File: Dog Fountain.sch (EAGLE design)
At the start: 19 parts, among them IC1 L298, J1 22-27-2021-02, J4 22-27-2021-02

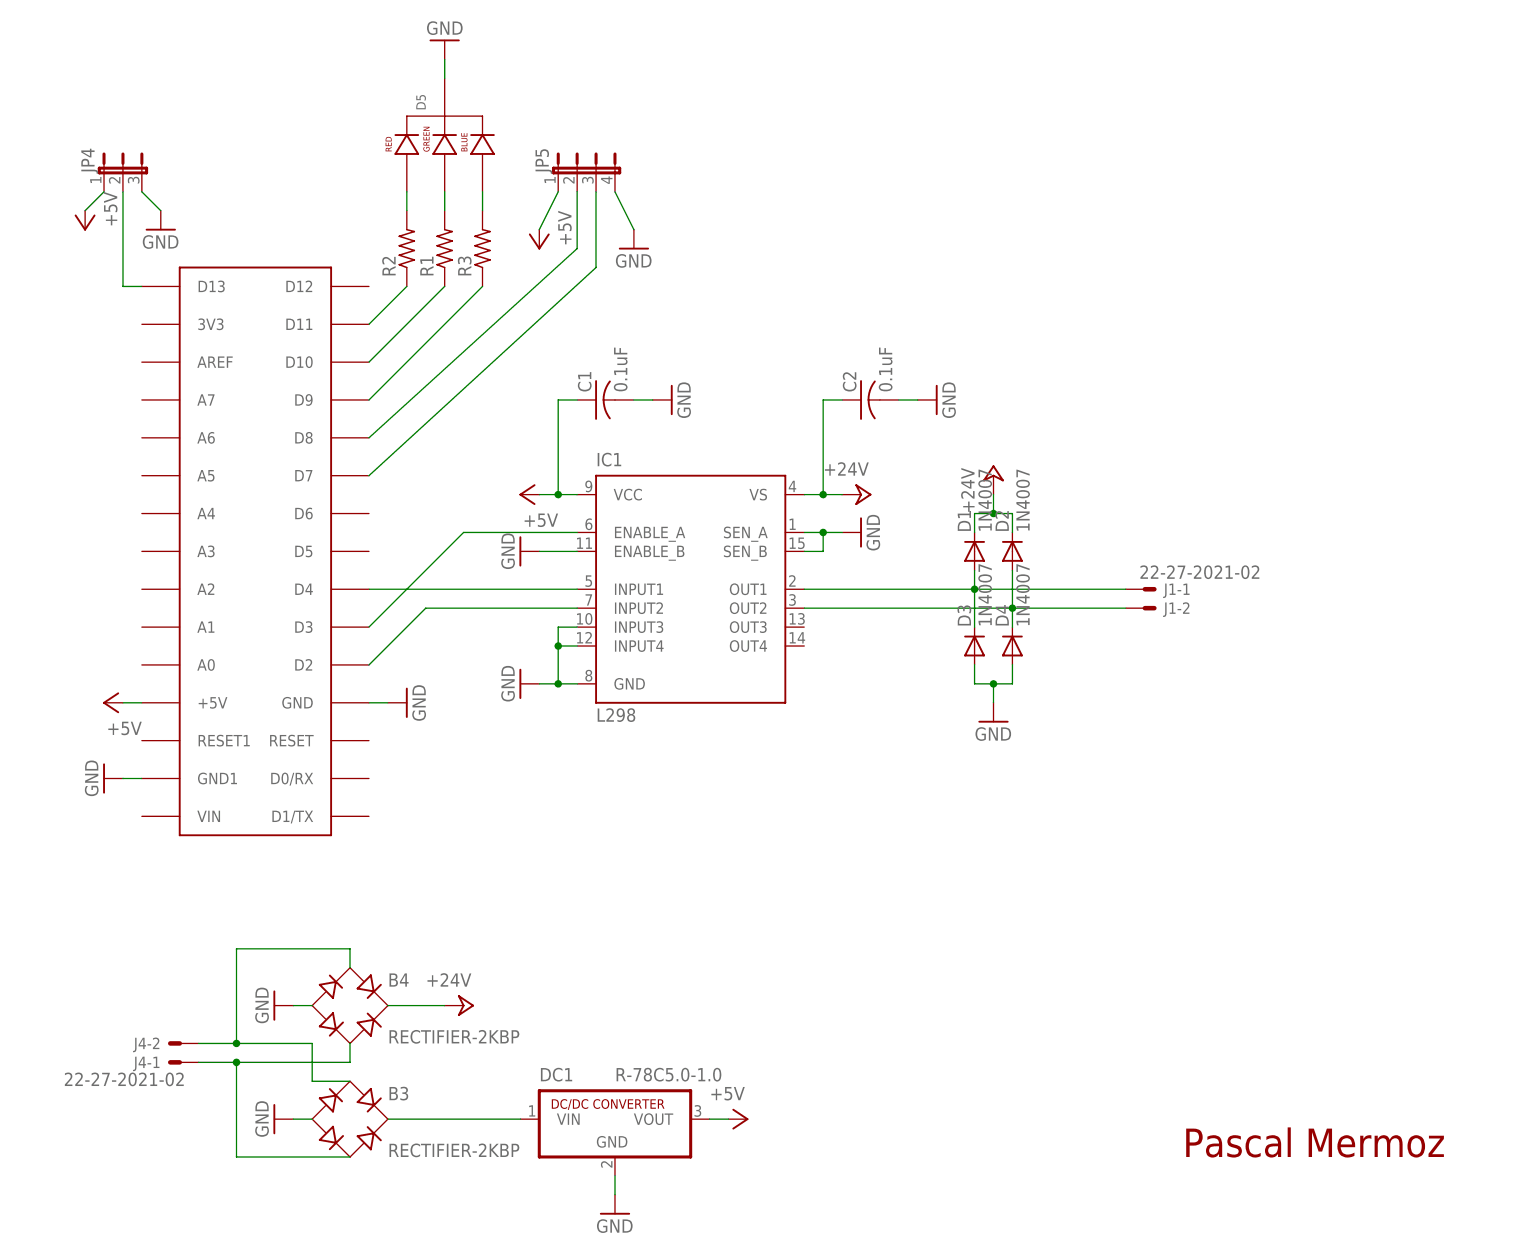
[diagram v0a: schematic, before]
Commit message: PCB board first test
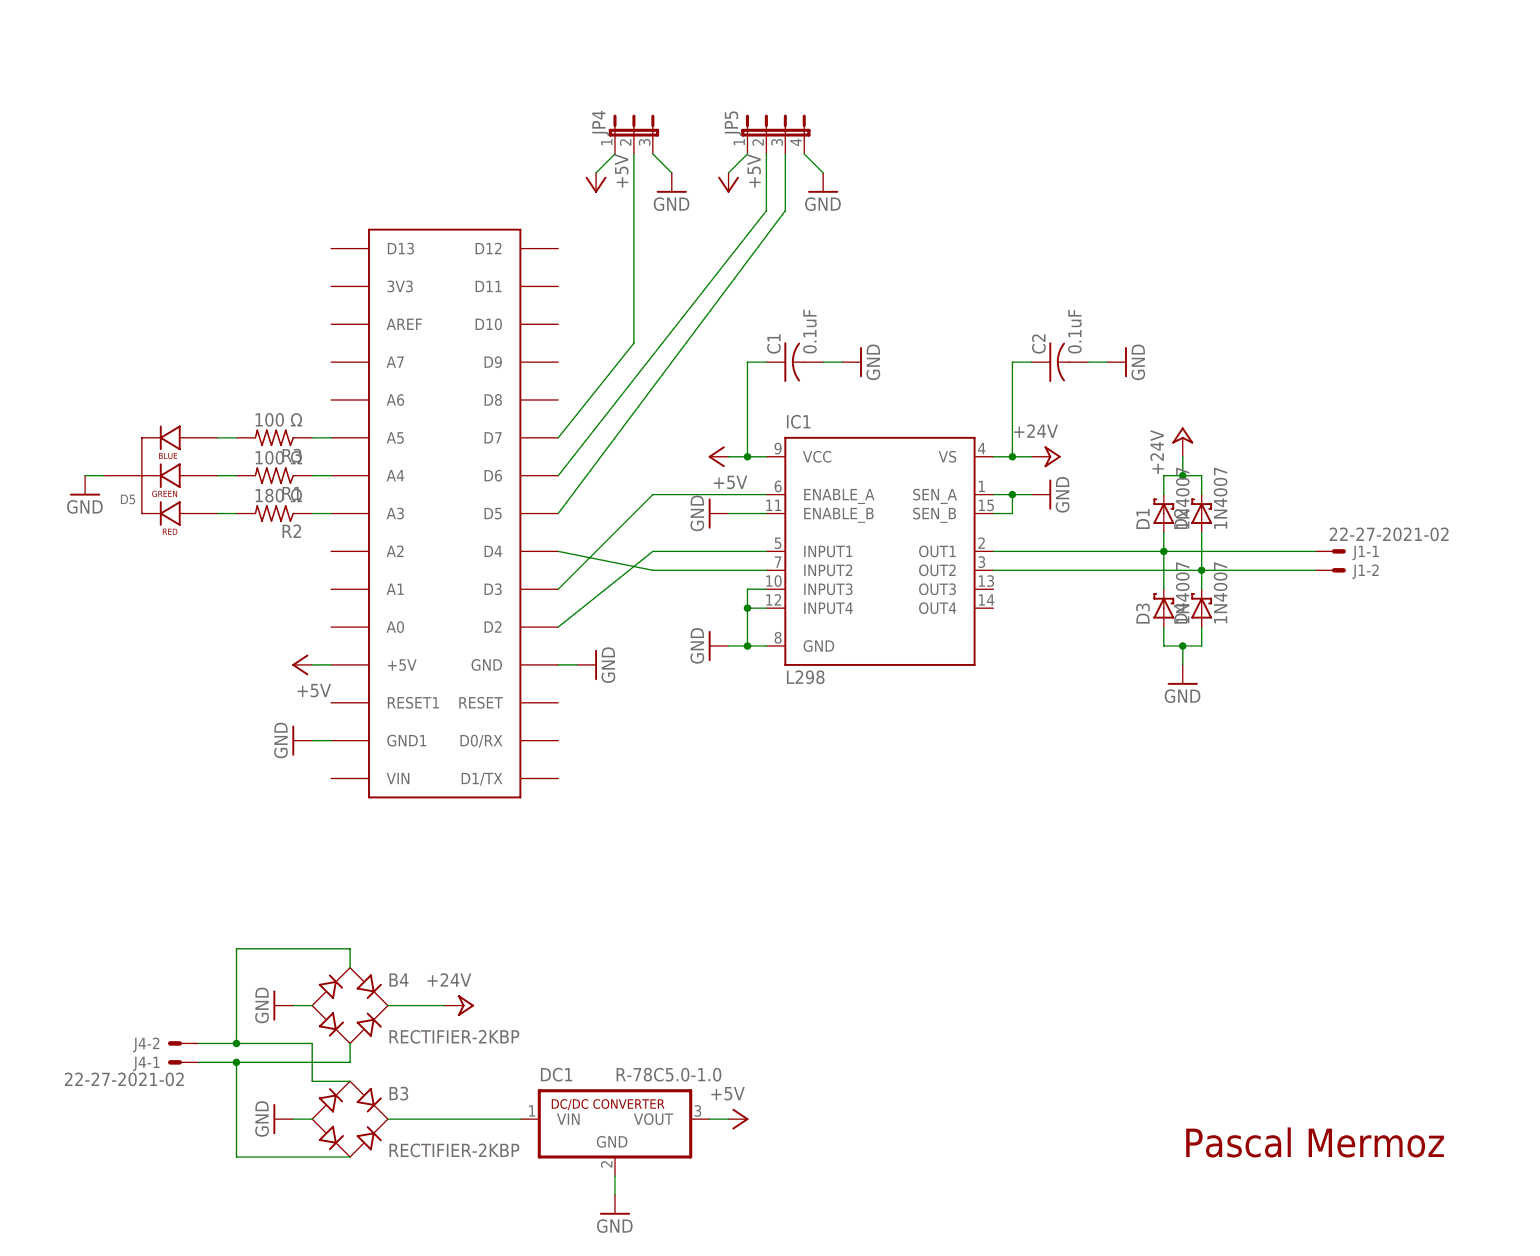
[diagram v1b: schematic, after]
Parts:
- D1, D2, D3, D4: device diode:DIODE-DO41-10 -> diode:1N5818-B
- R1, R3: value (none) -> 100 Ω
- R2: value (none) -> 180 Ω
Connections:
- net N$11: now also U$1.D7; no longer U$1.D13
- net N$12: now also U$1.D6; no longer U$1.D8
- net N$13: now also U$1.D5; no longer U$1.D7
- net N$14: now also U$1.A5; no longer U$1.D9
- net N$15: now also U$1.A4; no longer U$1.D10
- net N$16: now also U$1.A3; no longer U$1.D11
- net N$5: now also U$1.D2; no longer U$1.D4
- net N$8: now also U$1.D4; no longer U$1.D2
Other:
- moved on the sheet: C1, C2, D5, IC1, J1-1, J1-2, JP4, JP5, R1, R2, R3
